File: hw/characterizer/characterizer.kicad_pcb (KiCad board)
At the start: 4 copper layers, 217 parts, among them J1 1988820, J10 36-54-ND, J11 36-54-ND, J2 Conn_02x05_Odd_Even, J3 10118194-0001LF, J4 36-54-ND, J5 36-54-ND, J6 36-54-ND, J7 36-54-ND, J8 36-54-ND, J9 36-54-ND, Q1 BSS123, Q10 BSS123, Q11 FDMA008P20LZ, Q12 FDMA008P20LZ, Q13 BSS84, Q14 BSS123, Q15 BSS123, Q16 BSS123, Q17 FDMA008P20LZ, Q18 FDMA008P20LZ, Q19 PSMN7R0-30MLC,115, Q2 BSS123, Q20 BSS123, Q21 BSS84, Q22 BSS123, Q23 BSS123, Q24 BSS123, Q25 FDMA008P20LZ, Q26 FDMA008P20LZ, Q27 BSS84, Q28 BSS123, Q29 FDMA008P20LZ, Q3 FDMA008P20LZ, Q30 FDMA008P20LZ, Q31 FDMA008P20LZ, Q32 FDMA008P20LZ, Q33 FDMA008P20LZ, Q34 FDMA008P20LZ, Q35 FDMA008P20LZ, Q36 FDMA008P20LZ, Q4 FDMA008P20LZ, Q5 PSMN7R0-30MLC,115, Q6 BSS123, Q7 BSS84, Q8 BSS123, Q9 BSS123, U1 MIC5205-3.3, U10 AT30TS74, U11 TLV272CS-13, U12 TPS54719, U13 TLV272CS-13, U2 STM32F042K6T6, U3 74LVC2G04GW,125, U4 AT30TS74, U5 AT30TS74, U6 TLV272CS-13, U7 TPS54719, U8 TLV272CS-13, U9 AT30TS74, Y1 ABLS-8.000MHZ-B4-T

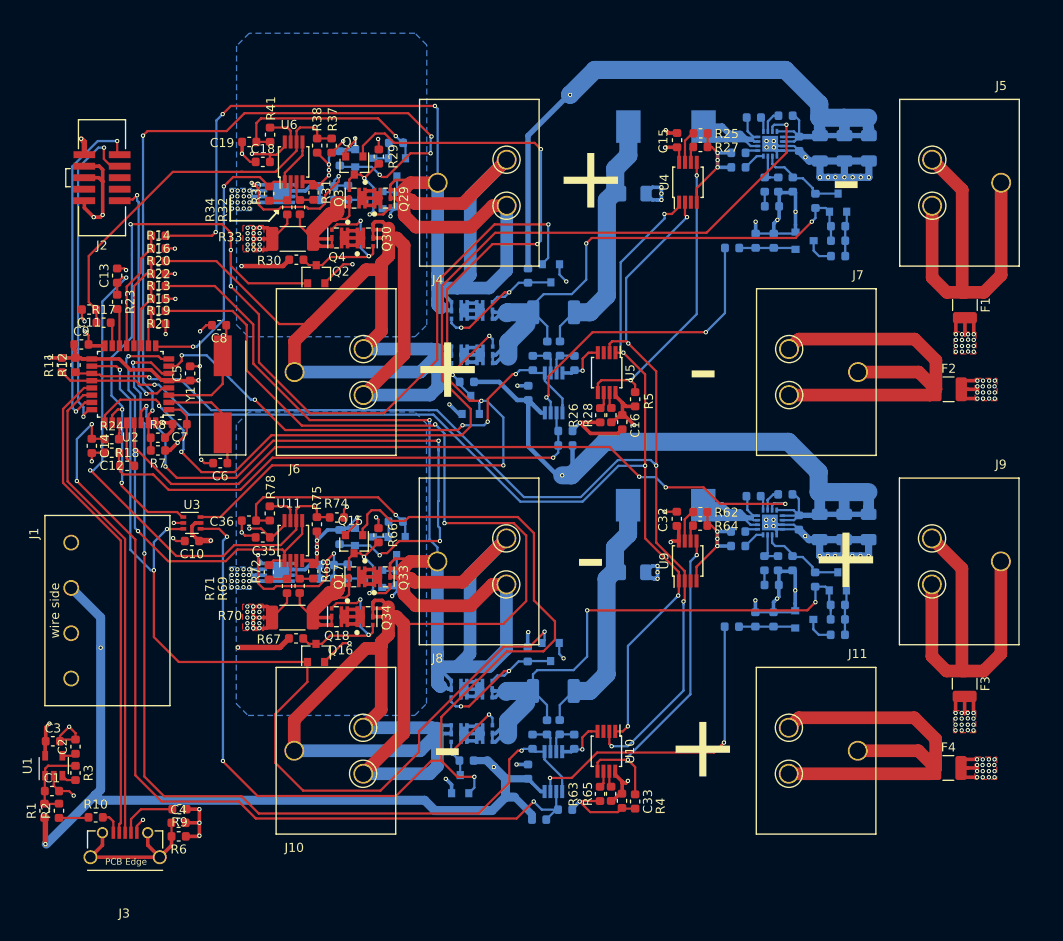
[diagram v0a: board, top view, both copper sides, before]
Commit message: layout as-ordered
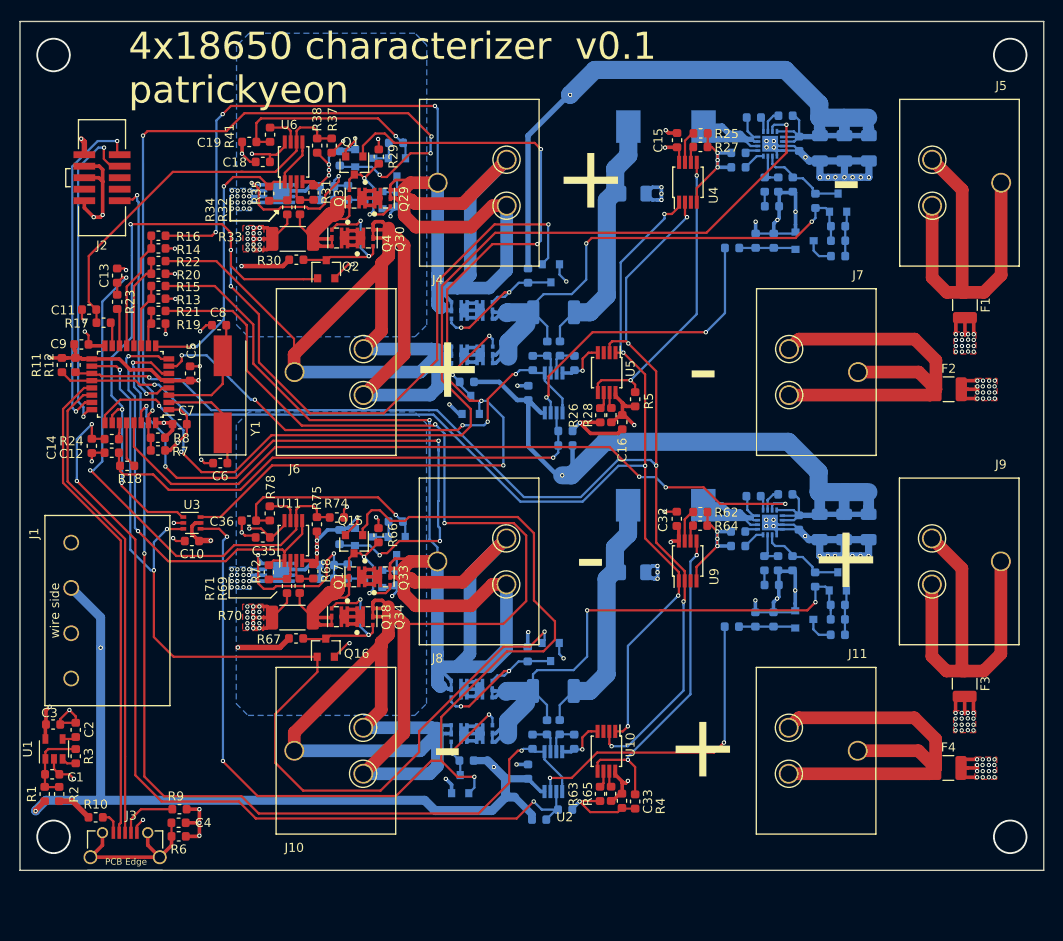
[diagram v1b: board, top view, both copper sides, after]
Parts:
- moved C2 1.85 mm to (129.2, 130.2)
- moved C3 1.85 mm to (126.7, 129.6)
- moved R2 1.85 mm to (127.3, 137.3)
- moved R3 1.85 mm to (129.2, 133.1)
- moved U1 1.85 mm to (126.8, 132.3)
- moved C1 1.85 mm to (126.5, 135.1)
- moved R1 1.85 mm to (125.7, 137.3)
- moved Q2 1.23 mm to (156.8, 79.3)
- moved Q16 1.22 mm to (156.8, 121.1)
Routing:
- net GND: track 315.5 -> 312.8 mm, vias 186 -> 190
- net +3V3: track 366.6 -> 368.7 mm
- net /pairA/DIR: track 113.2 -> 115.1 mm
- net +6V: track 500.2 -> 498.3 mm
- net /pairB/DIR: track 131.5 -> 132.4 mm
- net /mcu/VBAT1: track 181.3 -> 180.5 mm
- net +5V: track 3.29 -> 4.07 mm
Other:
- board outline added: 113 x 93.7 mm
- board text added: "4x18650 characterizer v0.1 patrickyeon"
